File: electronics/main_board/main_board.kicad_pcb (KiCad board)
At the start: 6 copper layers, 49.7 x 49.8 mm, 91 parts, among them U1 HUSB238A-BB001-QN16R, U10 TJA1051TK/3, U11 NTTFS5C454NL, U13 NTTFS5C454NL, U14 NTTFS5C454NL, U15 NTTFS5C454NL, U16 NTTFS5C454NL, U17 NTTFS5C454NL, U18 TJA1051TK/3, U2 LMR51420YDD, U3 TPS62933DRL, U4 GT-USB-7004N, U6 ESP32-S3-WROOM-1, U7 STM32G474VEH6, U8 DRV8323SRTA, U9 AFD01-S35FCA-00

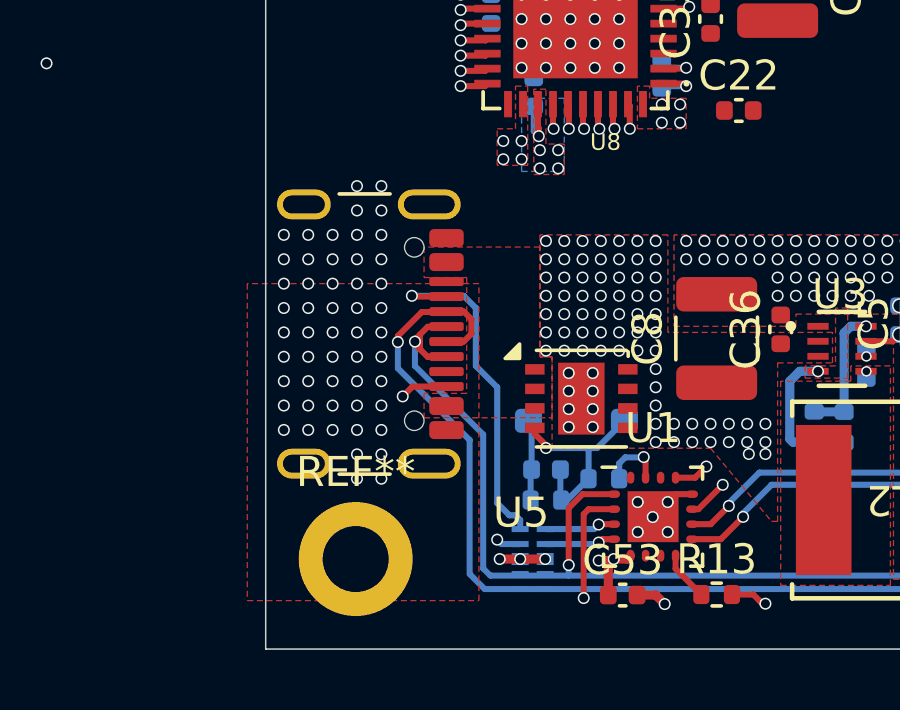
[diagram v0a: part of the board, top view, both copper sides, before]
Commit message: fix
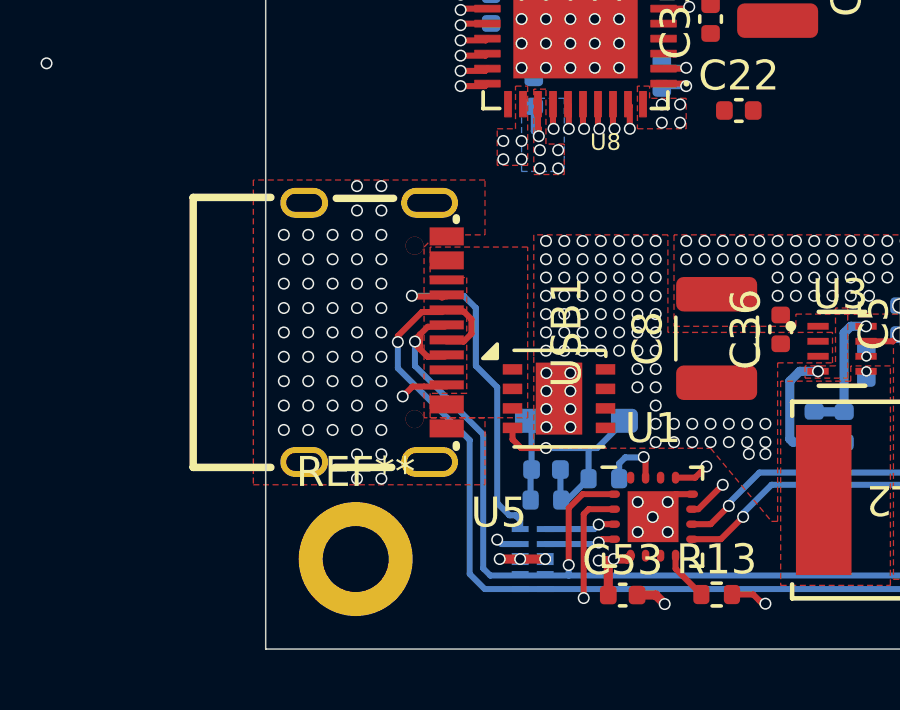
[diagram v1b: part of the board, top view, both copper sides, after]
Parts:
- removed U4: GT-USB-7004N, main_board:GT-USB-7004N
- added USB1: GT-USB-7004N, main_board:GT-USB-7004N, F.Cu at (117.7, 104.4)
- moved U5 0.74 mm to (123.7, 106.8)
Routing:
- net Net-(D4-A): track 7.08 -> 7.96 mm
- net VBUS: vias 131 -> 133
